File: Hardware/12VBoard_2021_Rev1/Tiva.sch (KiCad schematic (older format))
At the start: 2 parts

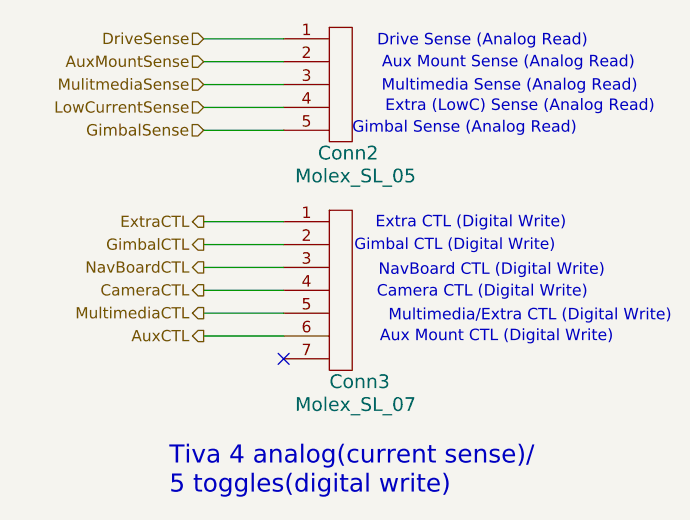
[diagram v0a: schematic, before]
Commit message: Added Component Values.
Added values to high side buck and
 footprints to components.
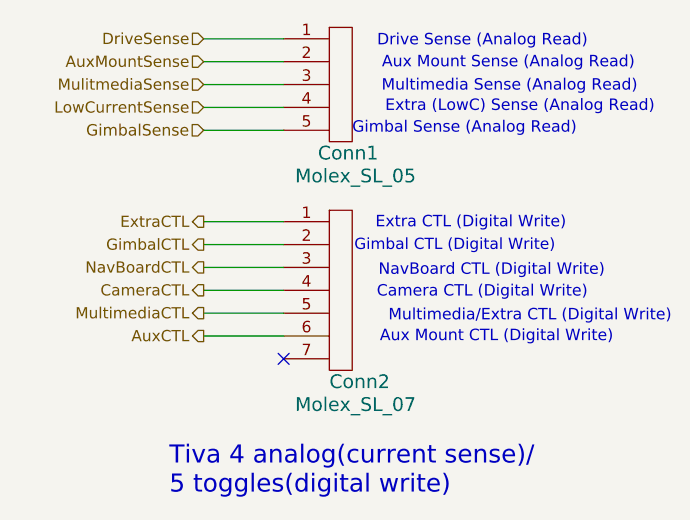
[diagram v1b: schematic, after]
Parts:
- renumbered Conn2 to Conn1, Conn3 to Conn2
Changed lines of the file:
@@
 	6150 2250 5800 2250
 $Comp
-L MRDT_Connectors:Molex_SL_05 Conn2
+L MRDT_Connectors:Molex_SL_05 Conn1
 U 1 1 5F976F73
 P 6350 1900
-F 0 "Conn2" H 6300 1850 60  0000 L CNN
+F 0 "Conn1" H 6300 1850 60  0000 L CNN
 F 1 "Molex_SL_05" H 6200 1750 60  0000 L CNN
 F 2 "MRDT_Connectors:MOLEX_SL_05_Horizontal" H 6350 1900 60  0001 C CNN
@@
 $EndComp
 $Comp
-L MRDT_Connectors:Molex_SL_07 Conn3
+L MRDT_Connectors:Molex_SL_07 Conn2
 U 1 1 5F97771C
 P 6350 2900
-F 0 "Conn3" H 6350 2850 60  0000 L CNN
+F 0 "Conn2" H 6350 2850 60  0000 L CNN
 F 1 "Molex_SL_07" H 6200 2750 60  0000 L CNN
 F 2 "MRDT_Connectors:MOLEX_SL_07_Horizontal" H 6350 3100 60  0001 C CNN

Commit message: Added Logic power circuits (High)
Added three smaller bucks for high current logic power and seprated acuation and logic pp
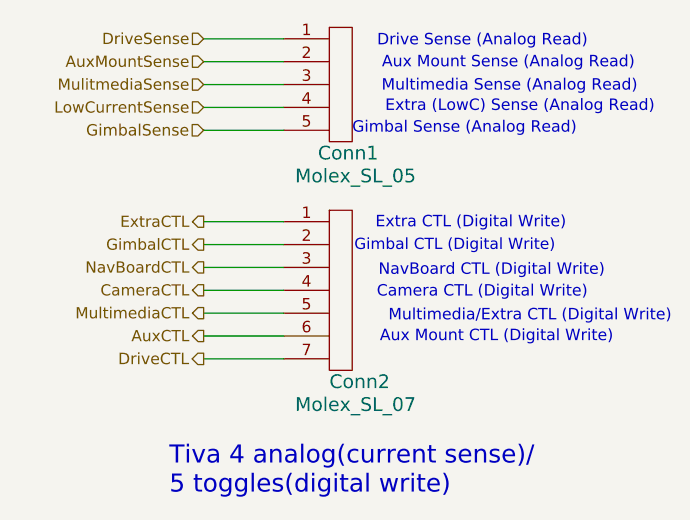
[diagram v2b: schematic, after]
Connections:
- net DriveCTL: now reaches Conn2.7
- no-connect marks 1 -> 0
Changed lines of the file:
@@
 Text Notes 6450 1872 0    50   ~ 0
 Gimbal Sense (Analog Read)
-NoConn ~ 6150 2850
+Text HLabel 5800 2850 0    50   Output ~ 0
+DriveCTL
+Wire Wire Line
+	6150 2850 5800 2850
 $EndSCHEMATC

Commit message: Layout Started
Board dimensions
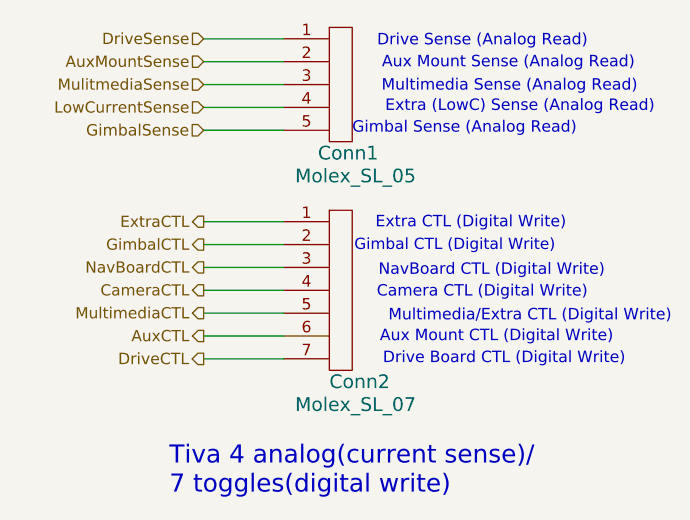
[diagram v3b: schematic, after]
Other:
- note added: "Drive Board CTL (Digital Write)"
- note added: "Tiva 4 analog(current sense)/ \n7 toggles(digital write)"
- note removed: "Tiva 4 analog(current sense)/ \n5 toggles(digital write)"
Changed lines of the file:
@@
 $Descr A4 11693 8268
 encoding utf-8
-Sheet 2 8
+Sheet 8 8
 Title ""
 Date ""
@@
 $EndDescr
 Text Notes 5650 3450 0    79   ~ 0
-Tiva 4 analog(current sense)/ \n5 toggles(digital write)
+Tiva 4 analog(current sense)/ \n7 toggles(digital write)
 Text Notes 7480 1490 2    50   ~ 0
 Drive Sense (Analog Read)
@@
 Wire Wire Line
 	6150 2850 5800 2850
+Text Notes 7645 2880 2    50   ~ 0
+Drive Board CTL (Digital Write)
 $EndSCHEMATC

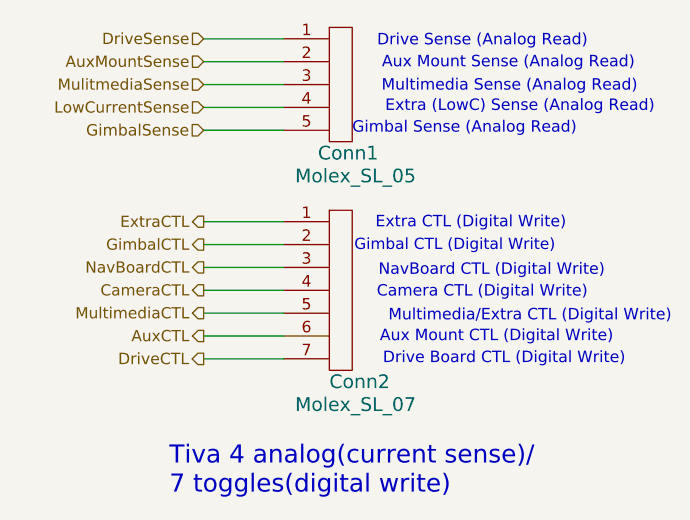
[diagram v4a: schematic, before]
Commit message: Checked H pins
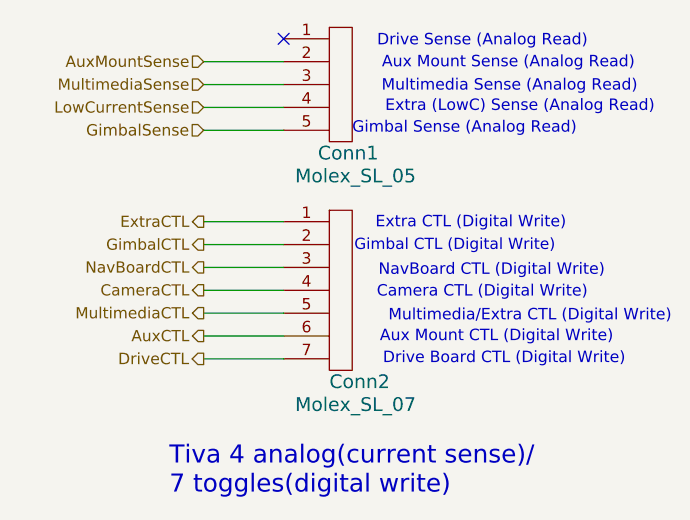
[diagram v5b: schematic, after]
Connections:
- net DriveSense: no longer names the net of Conn1.1
- net MulitmediaSense renamed MultimediaSense
- no-connect marks 0 -> 1
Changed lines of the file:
@@
 EESchema Schematic File Version 4
-LIBS:12VBoard_2021_Rev1-cache
 EELAYER 30 0
 EELAYER END
@@
 Text Notes 6459 2385 0    49   ~ 0
 Gimbal CTL (Digital Write)
-Text HLabel 5800 1450 0    49   Input ~ 0
-DriveSense
-Wire Wire Line
-	6150 1450 5800 1450
 Text HLabel 5800 1550 0    49   Input ~ 0
 AuxMountSense
@@
 	6150 1550 5800 1550
 Text HLabel 5800 1650 0    49   Input ~ 0
-MulitmediaSense
+MultimediaSense
 Wire Wire Line
 	6150 1650 5800 1650
@@
 Text Notes 7645 2880 2    50   ~ 0
 Drive Board CTL (Digital Write)
+NoConn ~ 6150 1450
 $EndSCHEMATC
